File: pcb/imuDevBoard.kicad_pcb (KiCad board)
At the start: 2 copper layers, 33 x 26 mm, 39 parts, among them J1 USB_C_Receptacle_USB2.0_16P, SW1 SW_Push, SW2 SW_SPDT, U1 RP2350A, U2 W25Q128JVS, U3 TLV75533PDBV, U4 ICM-42688-P, Y1 Crystal_GND24, 12MHz

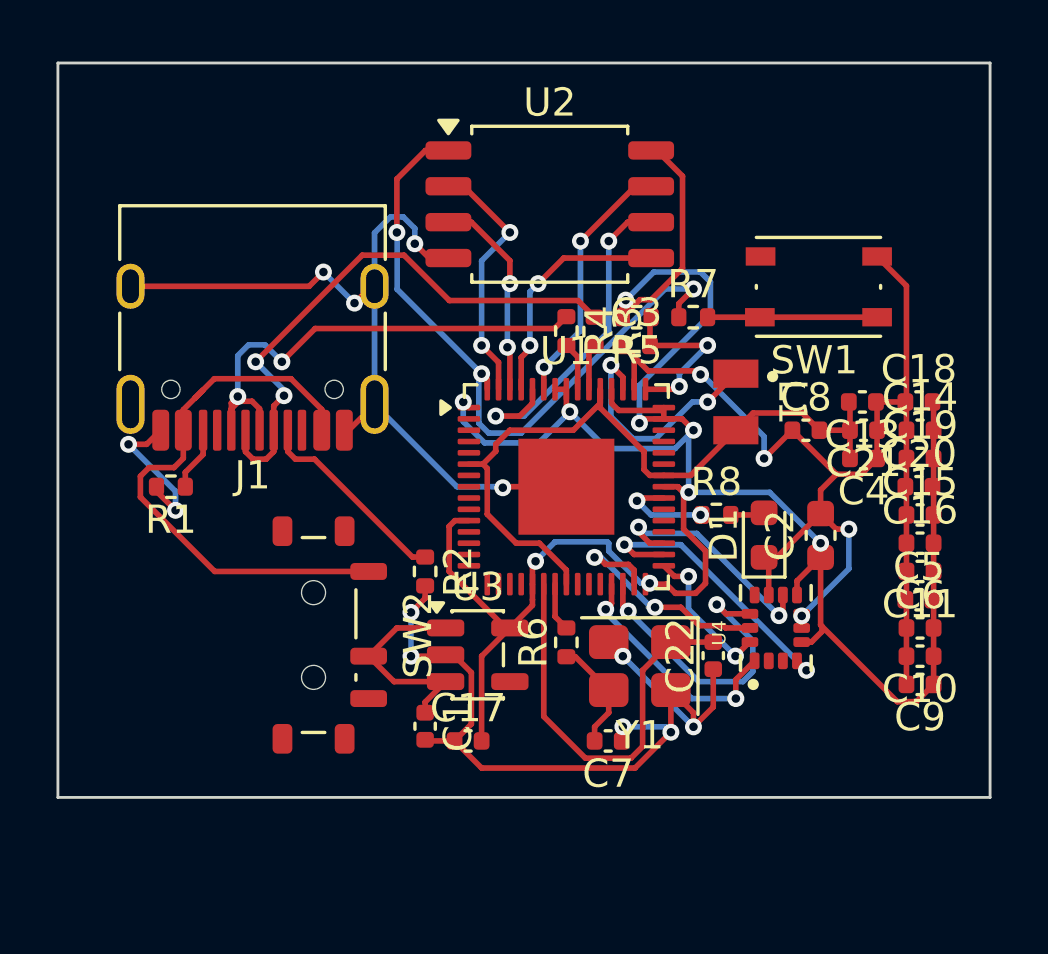
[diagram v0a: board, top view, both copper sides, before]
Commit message: fixed issues with pcb, see slack thread
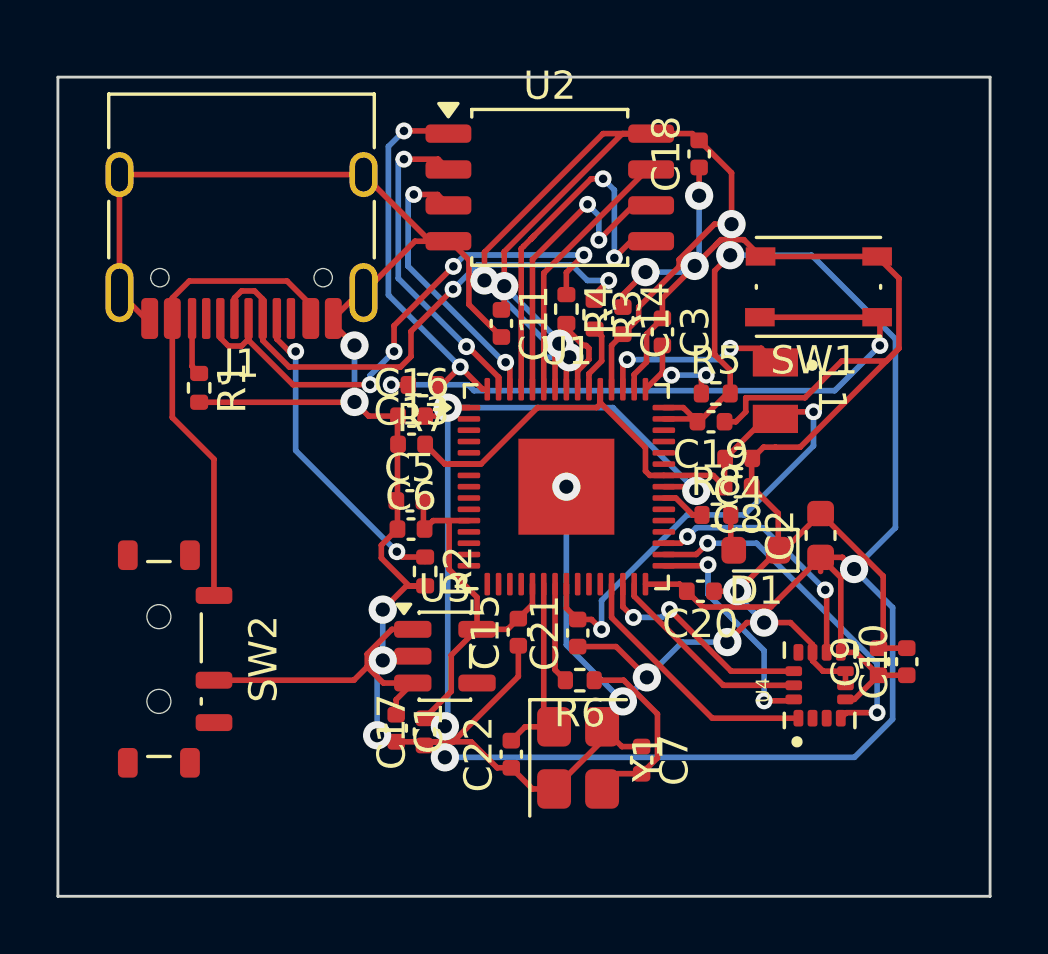
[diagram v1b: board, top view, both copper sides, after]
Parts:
- moved C16 18.6 mm to (63.5, 98.5)
- moved C5 18.4 mm to (63.5, 101.5)
- moved C6 18.4 mm to (63.5, 102.5)
- moved C11 17.2 mm to (66.7, 95.2), turned to -90 degrees
- moved C13 16.0 mm to (63.5, 99.5), turned to 0 degrees
- moved C15 14.8 mm to (67.3, 106.2), turned to 90 degrees
- moved C21 12.4 mm to (69.4, 106.2), turned to 90 degrees
- moved C18 11.7 mm to (73.7, 89.2), turned to 90 degrees
- moved C14 11.2 mm to (71.0, 95.1), turned to -90 degrees
- moved R7 9.88 mm to (63.9, 97.4), turned to 180 degrees
- moved C20 8.57 mm to (73.7, 104.7), turned to 180 degrees
- moved C22 7.96 mm to (67.0, 110.5)
- moved C19 7.51 mm to (74.1, 98.7), turned to 180 degrees
- moved SW2 5.54 mm to (54.6, 107.1)
- moved C4 4.42 mm to (75.1, 100.0)
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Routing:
- net +3V3: track 88.5 -> 147.5 mm, vias 9 -> 11
- net GND: track 107.8 -> 147.4 mm, vias 16 -> 14
- net Net-(R7-Pad2): track 6.00 -> 23.8 mm, vias 0 -> 2
- net Net-(U1-~{QSPI_SS}): track 23.9 -> 13.6 mm, vias 3 -> 2
- net Net-(U1-VREG_FB): track 26.2 -> 34.3 mm, vias 0 -> 2
- net Net-(U1-XIN): track 14.6 -> 6.92 mm
- net Net-(U1-QSPI_SD0): track 8.36 -> 13.7 mm
- net Net-(J1-CC1): track 7.16 -> 11.4 mm, vias 0 -> 2
- net Net-(U1-QSPI_SD1): track 9.06 -> 12.5 mm
- net Net-(SW2-B): track 7.99 -> 11.4 mm
- net Net-(SW2-A): track 20.3 -> 17.1 mm
- net Net-(U1-QSPI_SD2): track 7.36 -> 10.5 mm
- net Net-(U1-GPIO19): track 5.26 -> 8.29 mm
- net Net-(U1-GPIO17): track 10.8 -> 8.03 mm
- net Net-(C7-Pad2): track 4.00 -> 6.70 mm
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- removed copper zone on F.Cu, net GND
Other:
- board size 33 x 26 mm -> 33 x 29 mm
